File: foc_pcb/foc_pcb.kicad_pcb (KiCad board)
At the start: 4 copper layers, 73.7 x 50.8 mm, 59 parts, among them IC1 AS5600-ASOT, J1 MPU6050, J10 Conn_02x03_Top_Bottom, J12 10118193-0001LF, J2 Conn_01x02, J3 Conn_01x03, J4 power_supply, J5 XT60PW-M, J6 XT60PW-M, SW1 SW_Push, U1 DRV8313PWPR, U2 ATMEGA328P-AU, U3 BSS138-7-F, U4 BSS138-7-F, U5 CH340C, U7 BSS138-7-F, Y1 ABM3-16MHZ

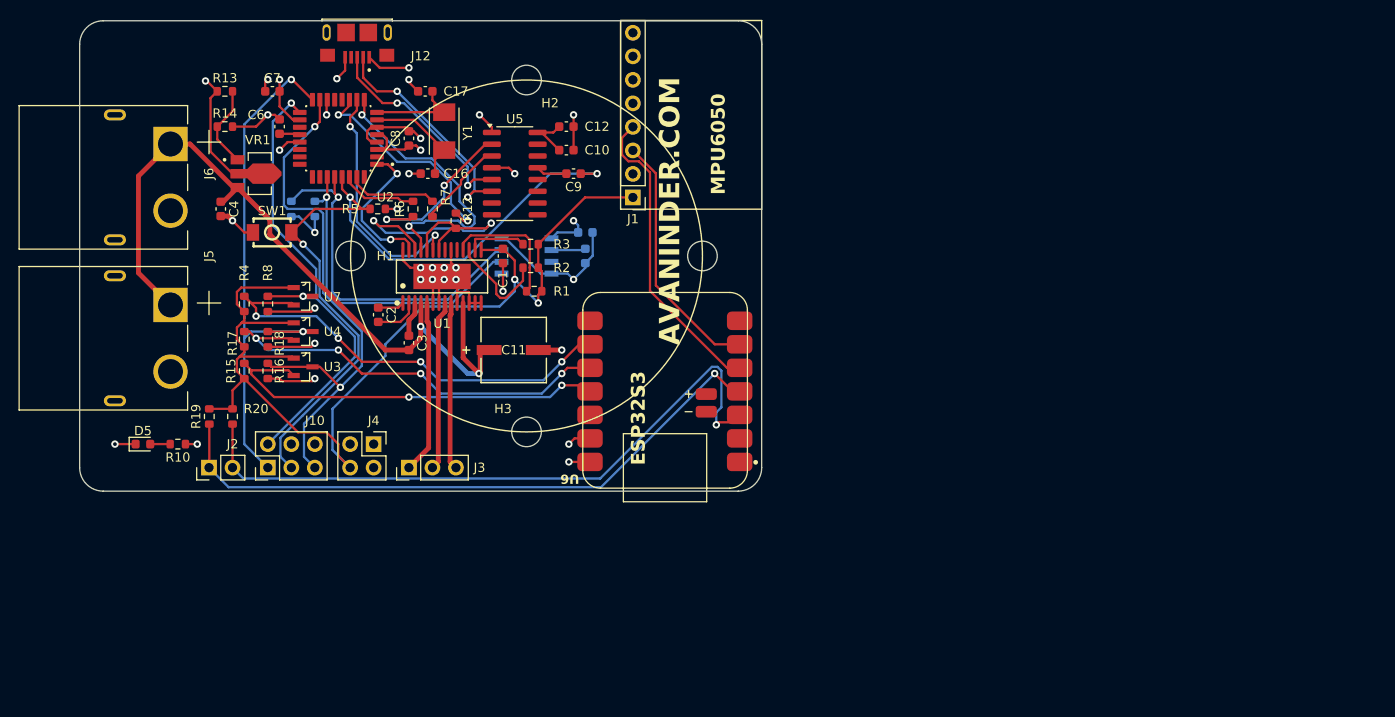
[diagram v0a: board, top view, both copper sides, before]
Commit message: V3 Intial Commit
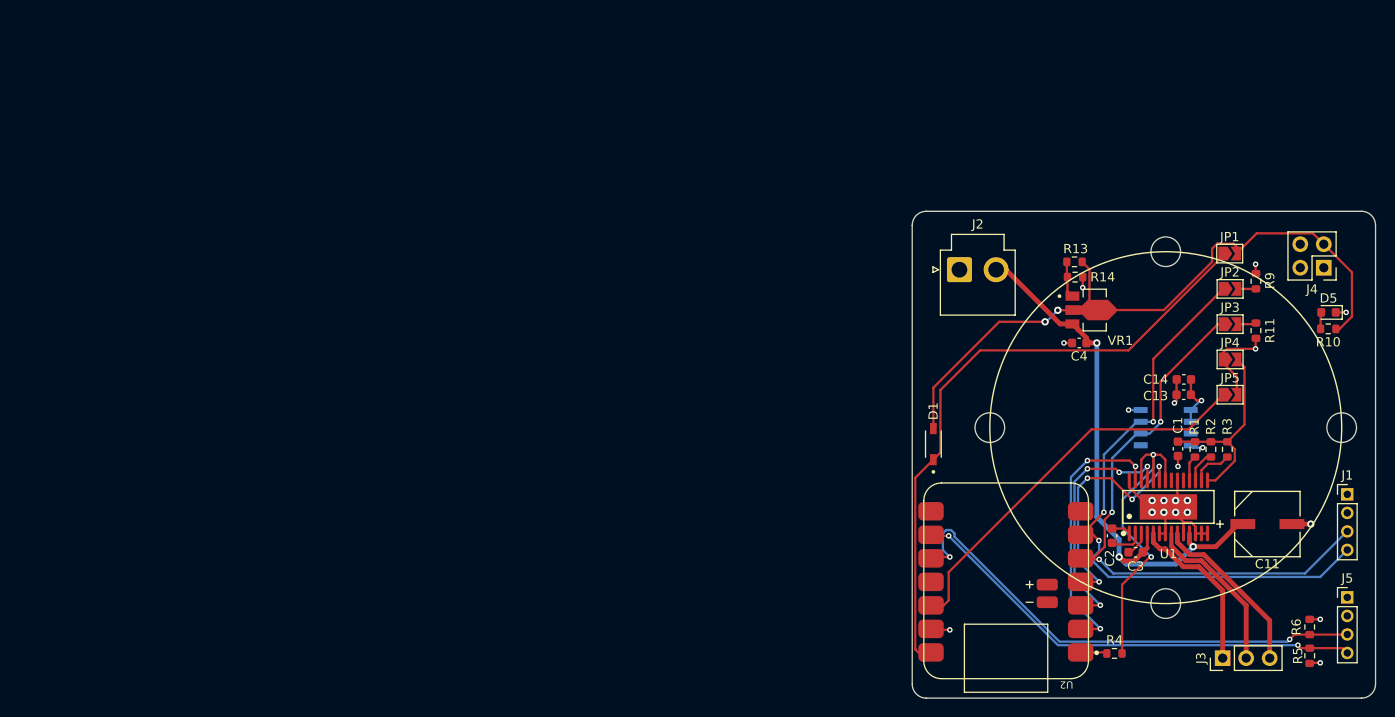
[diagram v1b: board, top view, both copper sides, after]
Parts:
- removed C10: 1nF, Capacitor_SMD:C_0603_1608Metric
- removed C12: 10nF, Capacitor_SMD:C_0603_1608Metric
- removed C16, C17: 22pF, Capacitor_SMD:C_0603_1608Metric
- removed C6, C7, C8, C9: 100nF, Capacitor_SMD:C_0603_1608Metric
- removed J10: Conn_02x03_Top_Bottom, Connector_PinHeader_2.54mm:PinHeader_2x03_P2.54mm_Vertical
- removed J12: 10118193-0001LF, usbMicroB:AMPHENOL_10118193-0001LF
- removed J6: XT60PW-M, XT60PW-M:AMASS_XT60PW-M
- removed R12, R15, R16, R17, R18, R19, R20, R8: 10k, Resistor_SMD:R_0603_1608Metric
- removed R7: 1k, Resistor_SMD:R_0603_1608Metric
- removed SW1: SW_Push, YTS-A011-2B:SW-SMD_L4.0-W3.0-LS4.6
- removed U3, U4, U7: BSS138-7-F, BSS138-7-F:SOT95P240X110-3N
- removed U5: CH340C, Package_SO:SOIC-16_3.9x9.9mm_P1.27mm
- removed U6: ~, XIAO-ESP32S3:MOUDLE14P-SMD-2.54-21X17.8MM
- removed Y1: ABM3-16MHZ, ABM3-16.000MHZ-B2-T:XTAL_ABM3-16.000MHZ-B2-T
- added D1: 1N5819HW-7-F, 1N5819HW-7-F:SOD3715X145N, F.Cu at (291.6, 143.5)
- added JP1: esp_diode_skip, Jumper:SolderJumper-2_P1.3mm_Open_TrianglePad1.0x1.5mm, F.Cu at (323.6, 122.9)
- added JP2: pullup_scl, Jumper:SolderJumper-2_P1.3mm_Open_TrianglePad1.0x1.5mm, F.Cu at (323.6, 126.7)
- added JP3: pullup_sda, Jumper:SolderJumper-2_P1.3mm_Open_TrianglePad1.0x1.5mm, F.Cu at (323.6, 130.6)
- added JP4: 3V3 DRV, Jumper:SolderJumper-2_P1.3mm_Open_TrianglePad1.0x1.5mm, F.Cu at (323.6, 134.4)
- added JP5: 3V3 ESP, Jumper:SolderJumper-2_P1.3mm_Open_TrianglePad1.0x1.5mm, F.Cu at (323.6, 138.2)
- C13, C14: moved to F.Cu
- J1: value MPU6050 -> IMU; footprint Connector_PinHeader_2.54mm:PinHeader_1x08_P2.54mm_Vertical -> Connector_PinHeader_2.00mm:PinHeader_1x04_P2.00mm_Vertical
- J2: value Conn_01x02 -> BATT_IN; footprint Connector_PinHeader_2.54mm:PinHeader_1x02_P2.54mm_Vertical -> Connector_JST:JST_VH_B2P-VH_1x02_P3.96mm_Vertical
- J5: value XT60PW-M -> ESP; footprint XT60PW-M:AMASS_XT60PW-M -> Connector_PinHeader_2.00mm:PinHeader_1x04_P2.00mm_Vertical
- R11, R9: value 4.7k -> 1k; moved to F.Cu
- R5: value 10k -> 4.7k
- R6: value 1k -> 4.7k
- U2: value ATMEGA328P-AU -> ~; footprint ATMEGA328P-AU:QFP80P900X900X120-32N -> XIAO-ESP32S3:MOUDLE14P-SMD-2.54-21X17.8MM
- moved J5 136.0 mm to (336.3, 160.1), turned to 0 degrees
- moved D5 128.8 mm to (334.3, 129.3), turned to 180 degrees
- moved R10 124.9 mm to (334.2, 131.1)
- moved R5 111.6 mm to (332.2, 166.4), turned to -90 degrees
- moved R6 106.8 mm to (332.2, 163.3)
- moved R9 104.5 mm to (326.4, 125.9), turned to -90 degrees
- moved J4 104.4 mm to (333.8, 124.5), turned to 180 degrees
- moved R11 102.5 mm to (326.4, 131.3)
- moved R4 101.3 mm to (311.1, 166.1), turned to 0 degrees
- moved C4 93.8 mm to (307.3, 132.6), turned to 180 degrees
- moved R13 93.6 mm to (306.8, 123.8), turned to 180 degrees
- moved R14 93.2 mm to (306.9, 125.5)
- moved VR1 91.4 mm to (308.6, 129.0)
- moved J3 90.3 mm to (322.8, 166.6)
- moved U2 89.2 mm to (308.3, 147.9)
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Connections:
- C1 pad 2: +3.3V -> /v3p3
- C13 pad 1: +5V -> +3.3V
- C14 pad 1: Net-(IC1-VDD3V3) -> +3.3V
- IC1 pad 1: +5V -> +3.3V
- IC1 pad 2: Net-(IC1-VDD3V3) -> +3.3V
- J1 pad 1: +3.3V -> GND
- J1 pad 2: GND -> +3.3V
- J1 pad 3: /esp_scl_1 -> /sda
- J1 pad 4: /esp_sda_1 -> /scl
- J2 pad 1: /esp_scl_0 -> GND
- J2 pad 2: /esp_sda_0 -> VCC
- J5 pad 1: VCC -> GND
- J5 pad 2: GND -> unconnected-(J5-Pin_2-Pad2)
- R1 pad 2: +3.3V -> /v3p3
- R11 pad 1: +5V -> +3.3V
- R11 pad 2: /sda -> Net-(JP3-B)
- R2 pad 2: +3.3V -> /v3p3
- R3 pad 2: +3.3V -> /v3p3
- R4 pad 1: +3.3V -> /en
- R4 pad 2: /esp_sck -> Net-(U1-EN1)
- R5 pad 1: /rst -> /esp_scl
- R5 pad 2: +5V -> +3.3V
- R6 pad 1: Net-(U5-TXD) -> /esp_sda
- R6 pad 2: /uRX -> +3.3V
- R9 pad 1: +5V -> +3.3V
- R9 pad 2: /scl -> Net-(JP2-B)
- U1 pad 15: +3.3V -> /v3p3
- U1 pad 22: /en -> Net-(U1-EN1)
- U1 pad 24: /en -> Net-(U1-EN1)
- U1 pad 26: /en -> Net-(U1-EN1)
- U2 pad 1: /in1 -> /en
- U2 pad 10: /in3 -> /esp_sda
- U2 pad 11: Net-(U2-PD7) -> unconnected-(U2-PA6_A10_D10_MOSI-Pad11)
- U2 pad 12: unconnected-(U2-PB0-Pad12) -> Net-(JP5-A)
- U2 pad 13: unconnected-(U2-PB1-Pad13) -> GND
- U2 pad 14: GND -> Net-(JP1-A)
- U2 pad 15: /mosi -> unconnected-(U2-BAT+-Pad15)
- U2 pad 16: /miso -> unconnected-(U2-BAT--Pad16)
- U2 pad 2: unconnected-(U2-PD4-Pad2) -> /in1
- U2 pad 3: GND -> /in2
- U2 pad 4: +5V -> /in3
- U2 pad 5: GND -> /sda
- U2 pad 6: +5V -> /scl
- U2 pad 7: /x1 -> unconnected-(U2-PB08_D6_TX-Pad7)
- U2 pad 8: /x2 -> unconnected-(U2-PB09_D7_RX-Pad8)
- U2 pad 9: /in2 -> /esp_scl
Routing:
- net +3.3V: track 114.2 -> 19.2 mm, vias 2 -> 5
- net /rst: track 83.7 -> 0.00 mm, vias 3 -> 0
- net /esp_sda_0: track 72.2 -> 0.00 mm, vias 1 -> 0
- net /esp_scl_0: track 68.8 -> 0.00 mm, vias 1 -> 0
- net Net-(JP1-A): track 0.00 -> 67.7 mm
- net /miso: track 60.9 -> 0.00 mm, vias 2 -> 0
- net /mosi: track 58.8 -> 0.00 mm, vias 2 -> 0
- net /esp_sda: track 0.00 -> 54.3 mm, vias 0 -> 2
- net /sck: track 53.9 -> 0.00 mm, vias 2 -> 0
- net /esp_scl: track 0.00 -> 50.2 mm, vias 0 -> 2
- net /esp_sck: track 48.9 -> 0.00 mm, vias 4 -> 0
- net GND: track 80.5 -> 33.6 mm, vias 24 -> 17
- net /esp_miso: track 45.4 -> 0.00 mm, vias 4 -> 0
- net /esp_mosi: track 44.7 -> 0.00 mm, vias 2 -> 0
- net Net-(JP5-A): track 0.00 -> 42.8 mm
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- added copper zone on In1.Cu, net +3.3V
- removed copper zone on In1.Cu, net +5V
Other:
- board size 73.7 x 50.8 mm -> 50 x 52.6 mm
- board text removed: "AVANINDER.COM"
- board text removed: "ESP32S3"
- board text removed: "GimbalFOC"
- board text removed: "MPU6050"
- board text removed: "v2.0"
